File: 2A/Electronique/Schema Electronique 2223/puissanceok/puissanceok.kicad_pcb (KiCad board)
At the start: 4 copper layers, 66 x 57 mm, 82 parts, among them J1001 Conn_UART, J101 Bat 2, J102 Bat 1, J103 AU, J104 Switch, J105 Conn_RPI, J106 Conn_Phidget_PS_Stepper_1, J107 Conn_Phidget_PS_Stepper_2, J108 Conn_Phidget_PS_Stepper_3, J109 Conn_Phidget_PS_Stepper_4, J110 Conn_01x02, J1101 Conn_UART, J111 Conn_GND, J112 Conn_GPIO_unused, J113 Conn_3.3V, J114 Conn_01x05, J115 Conn_01x05, J201 Conn_FDC, J401 Conn_FDC, J501 Conn_FDC, J701 Conn_FDC, J801 Conn_UART, J901 Conn_XL320, U301 LT1076CR-PBF, U601 LT1076CR-PBF, U901 74LVC2G241

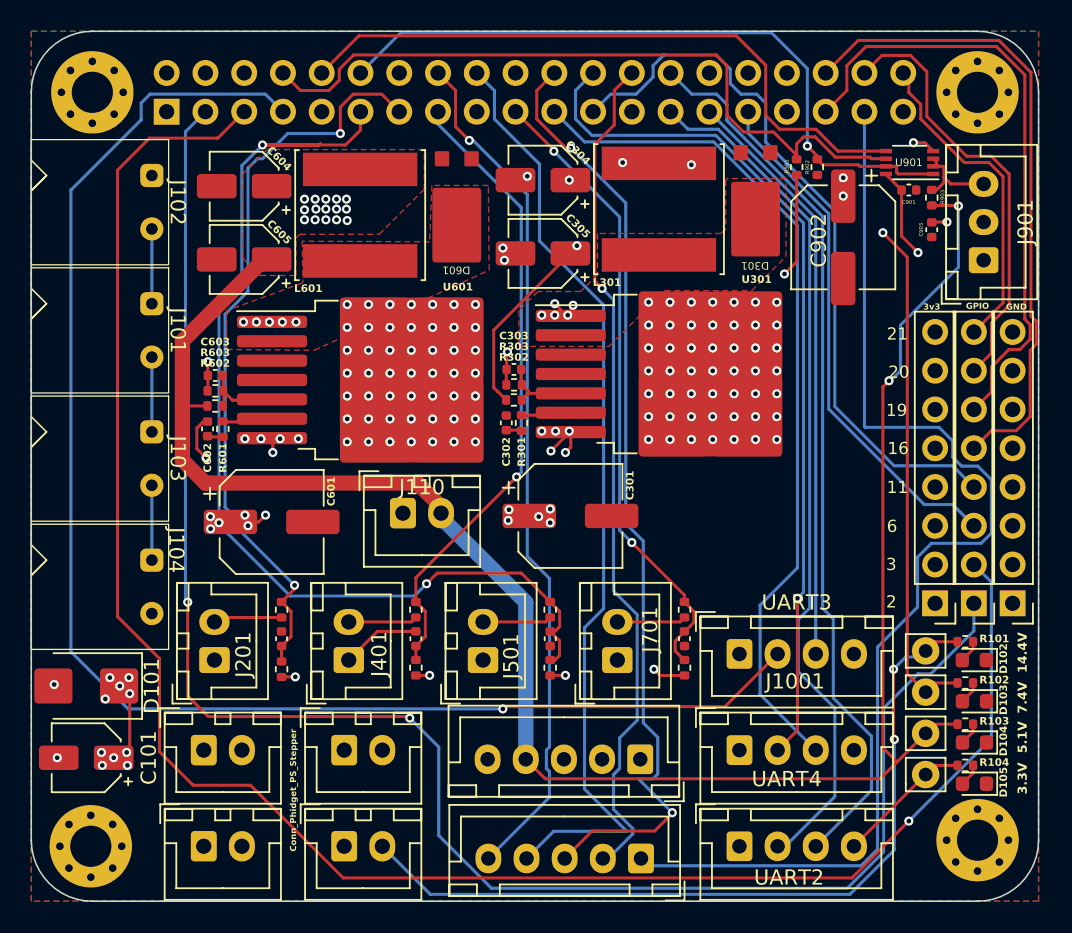
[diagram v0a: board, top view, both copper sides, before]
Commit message: update pcb
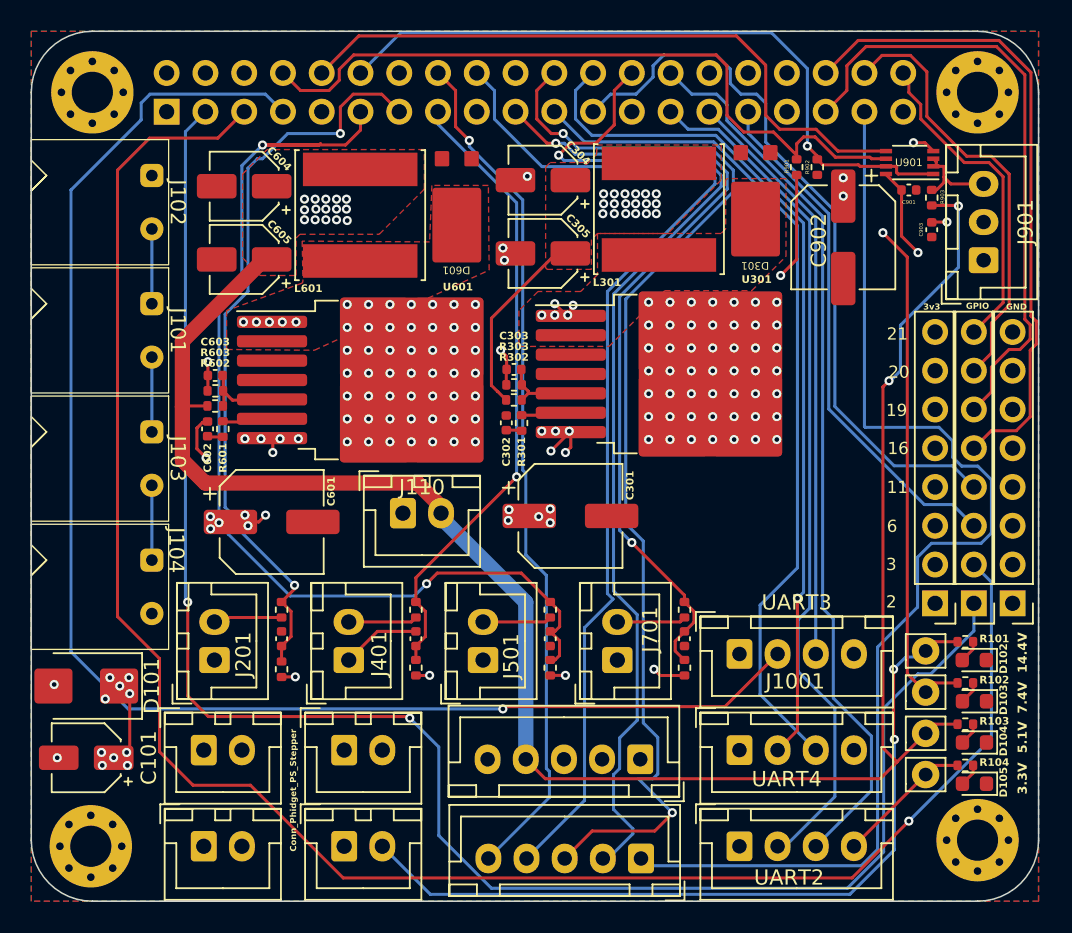
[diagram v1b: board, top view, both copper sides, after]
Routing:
- net /S3_color_sensor: track 55.8 -> 70.1 mm
- net /FDC_4: track 41.6 -> 53.2 mm
- net /S2_color_sensor: track 62.8 -> 74.0 mm
- net /S1_color_sensor: track 62.1 -> 69.6 mm
- net 7.4V: track 46.7 -> 47.4 mm, vias 8 -> 22
- added copper zone on F.Cu, net 7.4V
